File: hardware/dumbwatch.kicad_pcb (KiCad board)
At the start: 2 copper layers, 29.2 x 24.6 mm, 54 parts, among them J1 USB_C_Receptacle_USB2.0, J2 Programming Connector, J3 EINK, J4 JST PH, Q1 DMG3418L-7, Q2 NXV65UPR, U1 PIC18F27J53_ISS, U2 NCP115, U3 MCP73832T-2, Y1 32.768 kHz

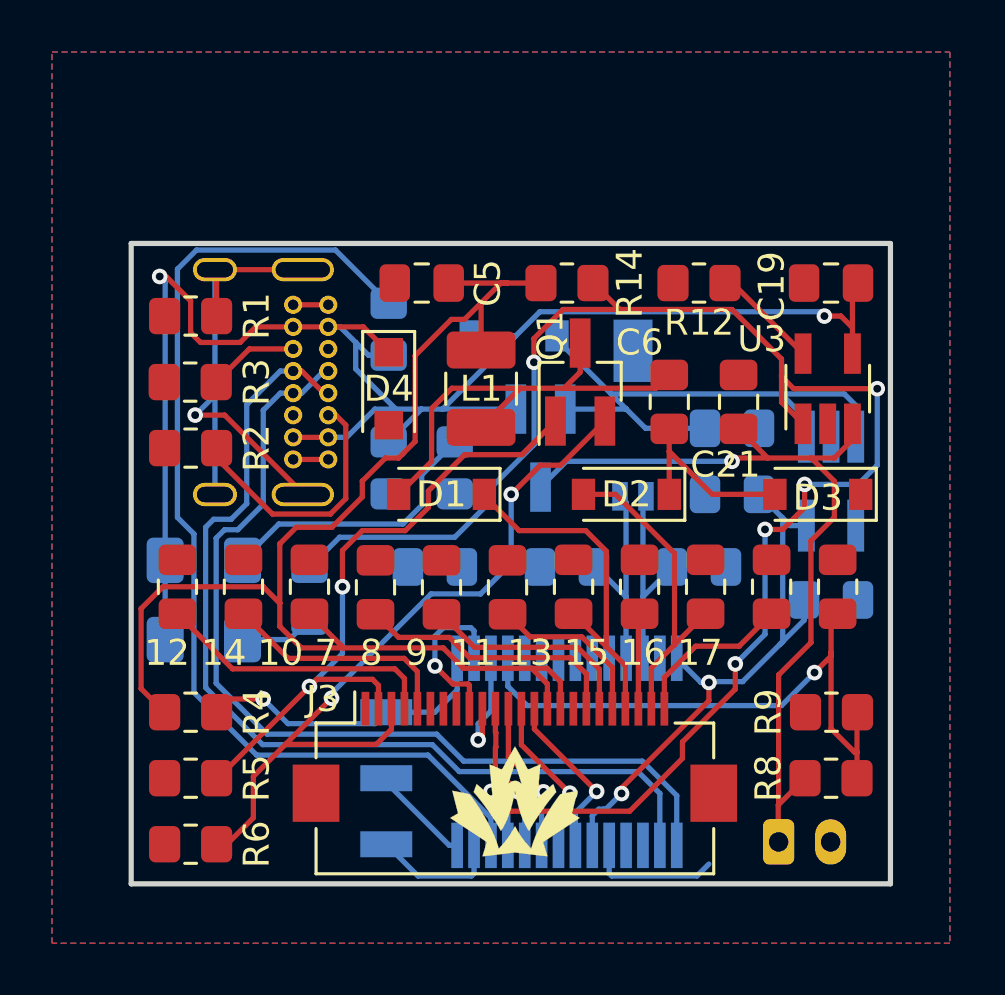
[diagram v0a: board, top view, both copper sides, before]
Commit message: PCB rev 1 complete
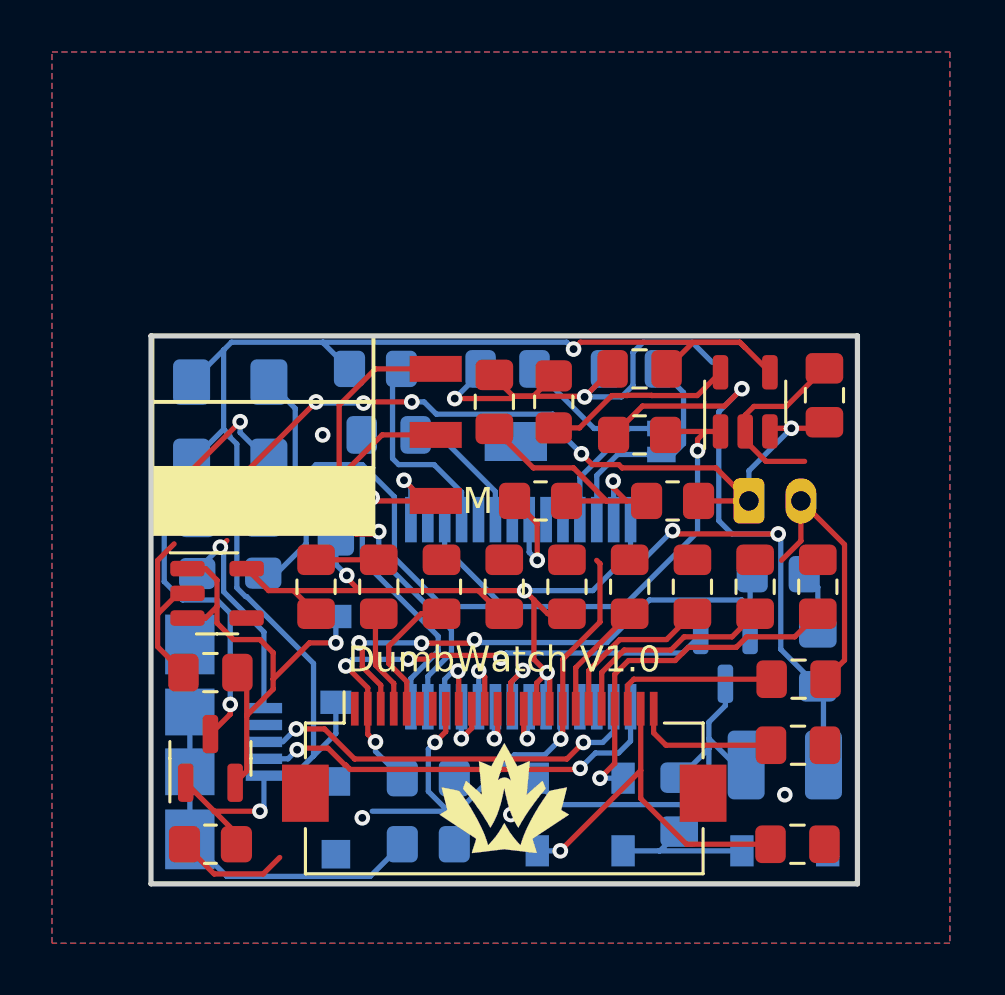
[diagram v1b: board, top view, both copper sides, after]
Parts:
- removed R2, R3: 5.1k, Resistor_SMD:R_0805_2012Metric_Pad1.20x1.40mm_HandSolder
- C18, C20, C4, J2, R11: moved to F.Cu
- C5, C6, D1, D2, D3, D4, L1, R1, R4, R5, R6: moved to B.Cu
- J1: value USB_C_Receptacle_USB2.0 -> USB_B_Micro; footprint Connector_USB:USB_C_Receptacle_GCT_USB4085 -> Connector_USB:USB_Micro-B_Amphenol_10104110_Horizontal
- Q1: footprint Package_TO_SOT_SMD:SOT-23_Handsoldering -> Package_TO_SOT_SMD:SOT-23; moved to B.Cu
- Q2: footprint Package_TO_SOT_SMD:SOT-23_Handsoldering -> Package_TO_SOT_SMD:SOT-23; moved to F.Cu
- U2: footprint Package_TO_SOT_SMD:TSOT-23-5_HandSoldering -> Package_TO_SOT_SMD:TSOT-23-5; moved to F.Cu
- U3: footprint Package_TO_SOT_SMD:SOT-23-5_HandSoldering -> Package_TO_SOT_SMD:SOT-23-5
- moved R6 24.9 mm to (126.5, 124.7), turned to 0 degrees
- moved U2 24.0 mm to (104.9, 125.5), turned to 0 degrees
- moved R1 22.3 mm to (113.0, 135.1)
- moved C18 22.2 mm to (104.6, 128.5), turned to 180 degrees
- moved C5 21.0 mm to (128.0, 128.0), turned to 90 degrees
- moved L1 18.6 mm to (126.7, 132.1), turned to 180 degrees
- moved Q2 17.4 mm to (104.6, 131.8), turned to 90 degrees
- moved D4 16.6 mm to (109.5, 134.1)
- moved C20 16.4 mm to (108.7, 125.2), turned to 90 degrees
- moved R11 16.0 mm to (104.6, 135.1), turned to 180 degrees
- moved C6 15.5 mm to (122.7, 133.6)
- moved C17 15.0 mm to (115.6, 118.1)
- moved D5 14.2 mm to (109.5, 128.0), turned to -90 degrees
- moved R9 13.8 mm to (117.3, 121.9)
- moved D2 13.8 mm to (118.9, 135.4)
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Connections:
- R1 pad 1: Net-(J1-PadS1) -> GND
- R1 pad 2: GND -> Net-(R1-Pad2)
- U1 pad 11: /OSC1 -> /OSC2
- U1 pad 12: /OSC2 -> /OSC1
- U1 pad 13: unconnected-(U1-Pad13) -> /BATT_SENS
- U1 pad 2: /BUSY -> unconnected-(U1-Pad2)
- U1 pad 25: /CHRG_STAT -> /RESET
- U1 pad 26: /USB_IN -> /BUSY
- U1 pad 3: /RESET -> /CHRG_STAT
- U1 pad 4: /BATT_SENS -> /USB_IN
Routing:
- net GND: track 7.84 -> 87.1 mm, vias 0 -> 10
- net /USB_IN: track 40.3 -> 7.35 mm
- net /CHRG_STAT: track 63.8 -> 34.6 mm, vias 6 -> 1
- net /D+: track 37.1 -> 14.8 mm, vias 0 -> 2
- net Net-(J1-PadS1): track 20.7 -> 0.00 mm, vias 1 -> 0
- net /D-: track 36.1 -> 16.4 mm, vias 0 -> 2
- net Net-(R1-Pad2): track 0.00 -> 16.8 mm
- net /ICSPCLK: track 5.00 -> 18.7 mm, vias 0 -> 1
- net /BATT_SENS: track 23.2 -> 11.0 mm
- net +3V3: track 73.1 -> 60.9 mm, vias 2 -> 6
- net +BATT: track 32.4 -> 43.8 mm, vias 1 -> 7
- net /ICSPDAT: track 3.89 -> 14.9 mm, vias 0 -> 1
- net Net-(J1-PadA5): track 10.2 -> 0.00 mm
- net /E-Ink Display/RESE: track 29.4 -> 21.1 mm, vias 2 -> 3
- net Net-(C12-Pad1): track 10.9 -> 3.82 mm
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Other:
- board size 29.2 x 24.6 mm -> 27.2 x 21.1 mm
- board text added: "+"
- board text added: "C"
- board text added: "DumbWatch V1.0"
- board text added: "M"
- board text added: "P"
- board text removed: "12 14 10 7 8 9 11 13 15 16 17"
- board text removed: "DumbWatch V1.0 Jack C"
